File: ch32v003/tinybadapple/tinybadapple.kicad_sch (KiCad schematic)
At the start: 9 parts, among them J1 USB_C_Receptacle_USB2.0, U1 RS3236-3.3YUTDN4, U2 ZD25WQ16BUIGR, U3 CH32V003F4U6

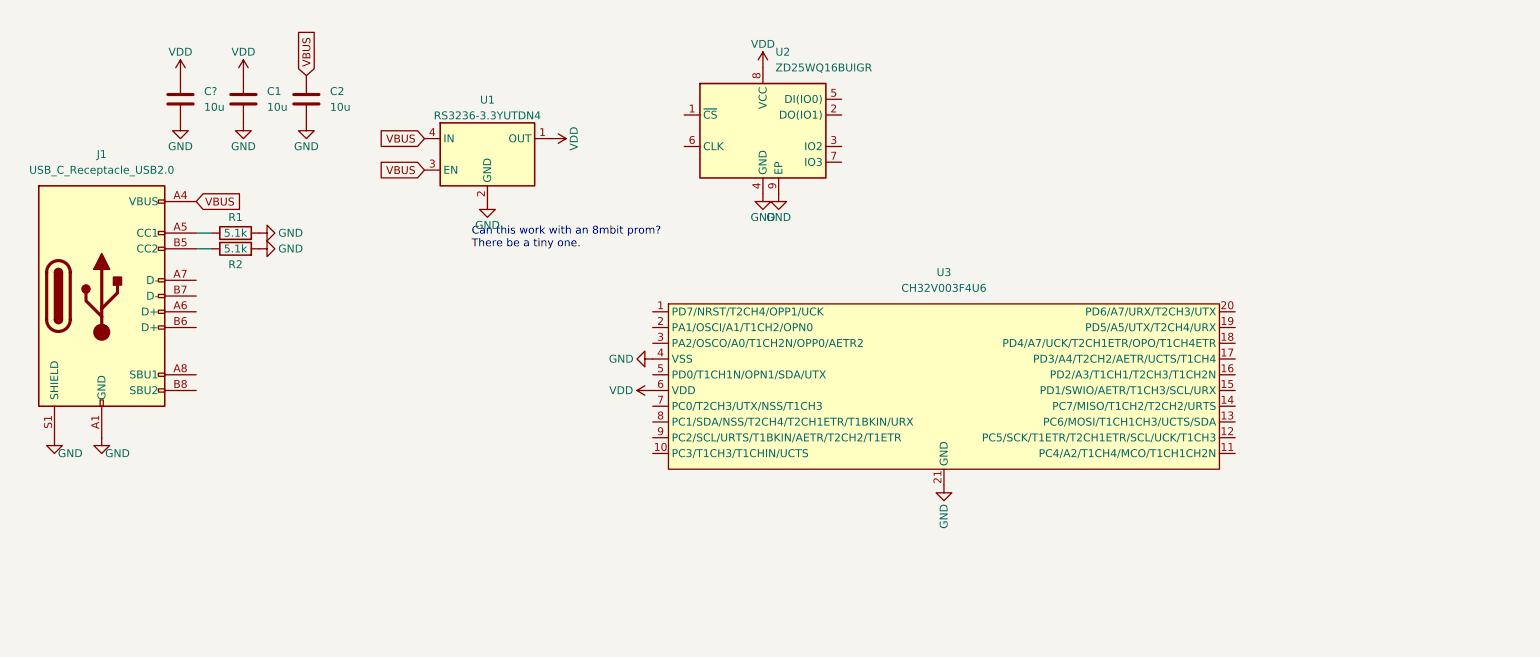
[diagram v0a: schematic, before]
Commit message: Bump versions.
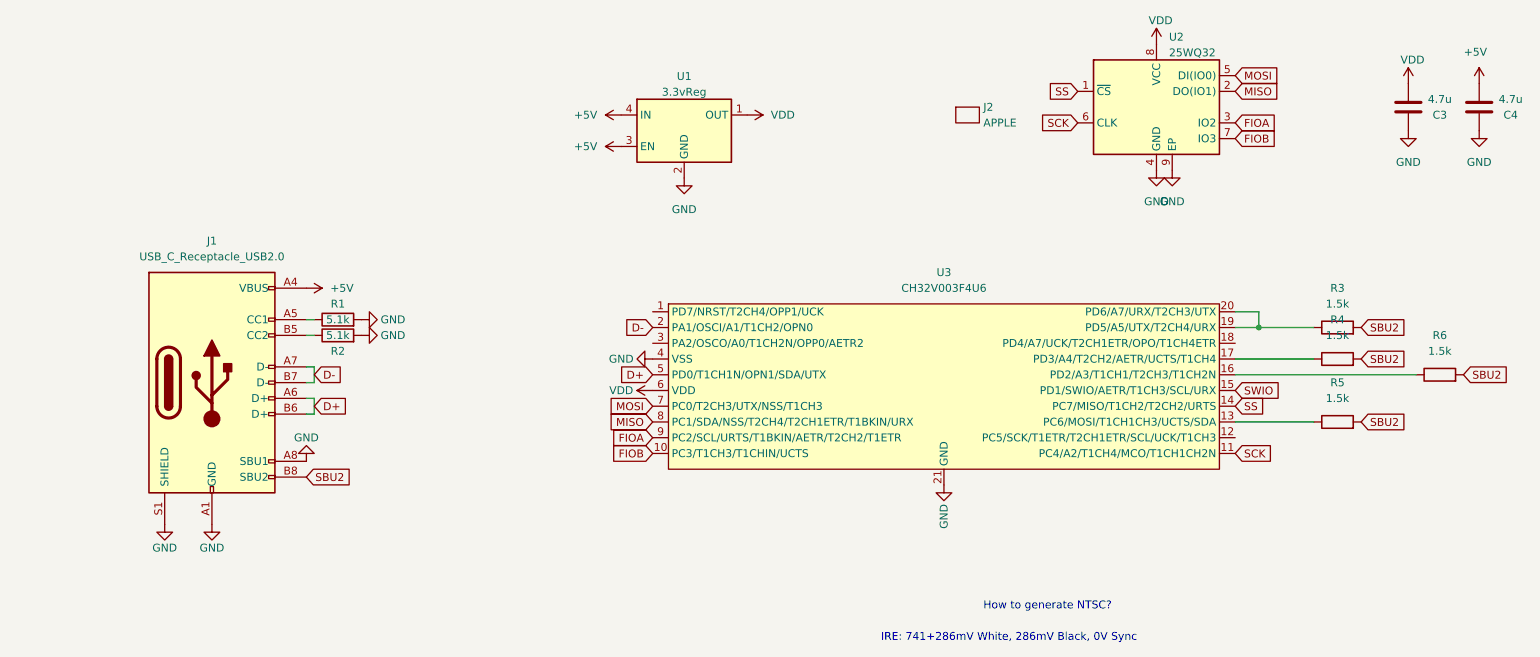
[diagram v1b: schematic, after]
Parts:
- removed C1, C2, C?: 10u, Capacitor_SMD:C_0402_1005Metric, symbol Device:C
- removed U1: RS3236-3.3YUTDN4, cnhardware:xdfn-reg, symbol Regulator_Linear:NCP115AMX250TCG
- added C3, C4: 4.7u, Resistor_SMD:R_0402_1005Metric, symbol Device:C
- added J2: APPLE, artwork:apple, symbol artwork:artwork
- added R3, R4, R5, R6: 1.5k, Resistor_SMD:R_0402_1005Metric, symbol Device:R
- added U1: 3.3vReg, cnhardware:xdfn-reg, symbol Regulator_Linear:NCP115AMX120TCG
- R1, R2: LCSC C105872 -> C25905
- U2: value ZD25WQ16BUIGR -> 25WQ32; footprint Package_SON:SON-8-1EP_3x2mm_P0.5mm_EP1.4x1.6mm -> cnhardware:USON8-LINE(2x3); LCSC C2983691 -> C5258281
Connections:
- net GND: now also J1.A8 (SBU1), C3.1, C4.1, U1.2 (GND), U1.5 (GND)
- net VDD: now also C3.2, U1.1 (OUT)
- net D+: now reaches J1.A6 (D+)
- net D+: now also J1.B6 (D+), U3.5 (PD0/T1CH1N/OPN1/SDA/UTX)
- net D-: now reaches J1.A7 (D-)
- net D-: now also J1.B7 (D-), U3.2 (PA1/OSCI/A1/T1CH2/OPN0)
- net SBU2: now reaches J1.B8 (SBU2)
- net SBU2: now also R3.2, R4.2, R5.2, R6.2
- net FIOB: now reaches U3.10 (PC3/T1CH3/T1CHIN/UCTS)
- net FIOB: now also U2.7 (IO3)
- net SCK: now reaches U3.11 (PC4/A2/T1CH4/MCO/T1CH1CH2N)
- net SCK: now also U2.6 (CLK)
- net at U3.13 (PC6/MOSI/T1CH1CH3/UCTS/SDA): now also R5.1
- net SS: now reaches U3.14 (PC7/MISO/T1CH2/T2CH2/URTS)
- net SS: now also U2.1 (~{CS})
- net SWIO: now reaches U3.15 (PD1/SWIO/AETR/T1CH3/SCL/URX)
- net at U3.16 (PD2/A3/T1CH1/T2CH3/T1CH2N): now also R6.1
- net at U3.17 (PD3/A4/T2CH2/AETR/UCTS/T1CH4): now also R4.1
- net at U3.19 (PD5/A5/UTX/T2CH4/URX): now also U3.20 (PD6/A7/URX/T2CH3/UTX), R3.1
- net MOSI: now reaches U3.7 (PC0/T2CH3/UTX/NSS/T1CH3)
- net MOSI: now also U2.5 (DI(IO0))
- net MISO: now reaches U3.8 (PC1/SDA/NSS/T2CH4/T2CH1ETR/T1BKIN/URX)
- net MISO: now also U2.2 (DO(IO1))
- net FIOA: now reaches U3.9 (PC2/SCL/URTS/T1BKIN/AETR/T2CH2/T1ETR)
- net FIOA: now also U2.3 (IO2)
- net VBUS renamed +5V
- net +5V: now also C4.2, U1.3 (EN), U1.4 (IN)
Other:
- note added: "How to generate NTSC?"
- note added: "IRE: 741+286mV White, 286mV Black, 0V Sync"
- note removed: "Can this work with an 8mbit prom? There be a tiny one."
